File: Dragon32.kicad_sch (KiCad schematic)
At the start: 81 parts, among them IC1 74HCT273, IC10 74HCT32, IC11 74LS123N, IC12 LM1889N, IC15 CD4053, IC2 MC6847, IC3 74HCT00, IC4 74HCT20, IC5 74HCT86, IC6 74HCT393, IC7 74ALS74N, IC8 74HCT393, IC9 74HCT390, J1 Board Interconnect Male, J2 Video Output, J3 YUV Output, J4 S-Video Test, U1 74AHC1G04, U2 TS971, Y1 4.433619MHz

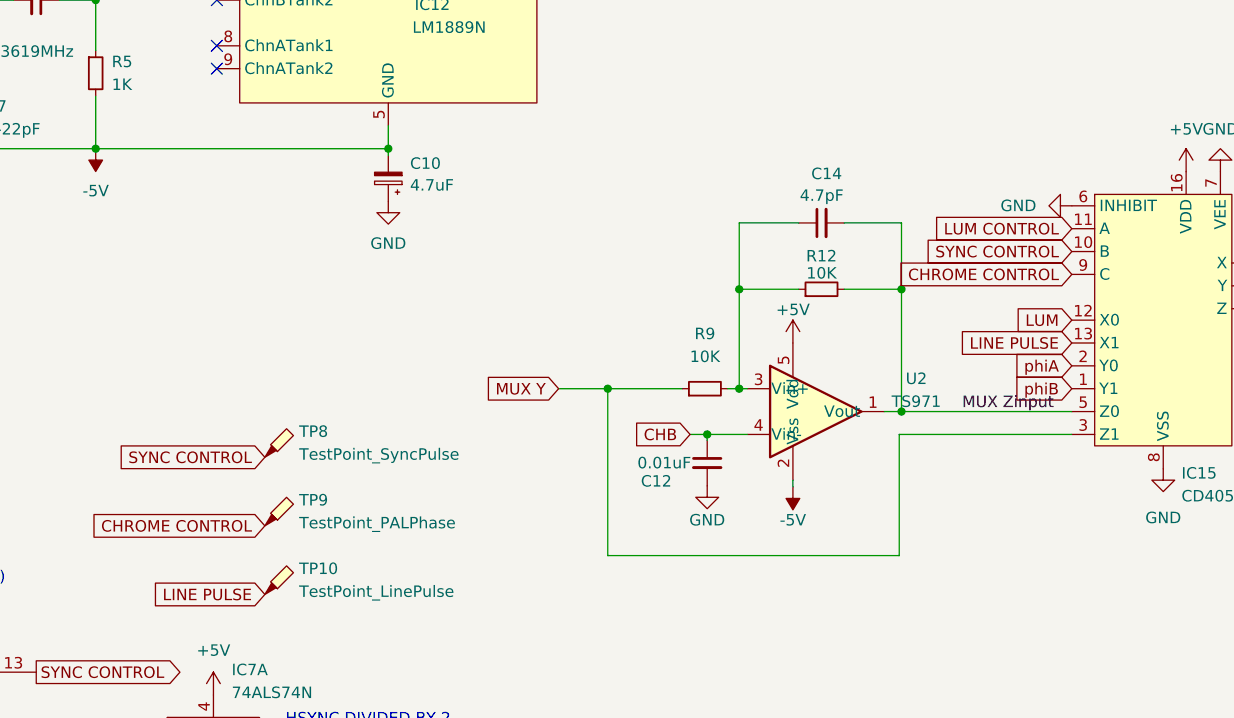
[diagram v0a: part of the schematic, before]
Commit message: refinement
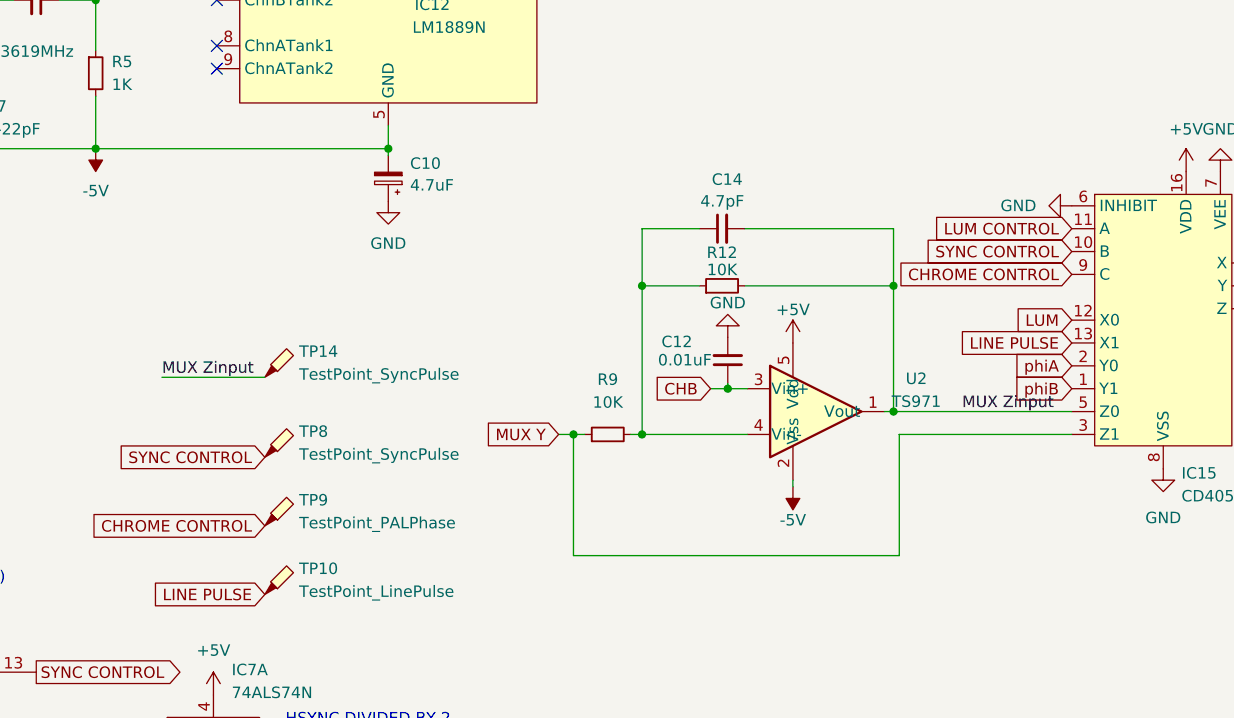
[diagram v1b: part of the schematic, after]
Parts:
- added TP14: TestPoint_SyncPulse, TestPoint:TestPoint_Pad_D1.0mm, symbol Connector:TestPoint_Probe
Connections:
- net CHB: now also U2.3 (Vin+); no longer U2.4 (Vin-)
- net MUX Zinput: now also TP14.1
- net at C14.1, R12.1, R9.2: now also U2.4 (Vin-); no longer U2.3 (Vin+)
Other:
- moved on the sheet: C12, C14, R12, R9
